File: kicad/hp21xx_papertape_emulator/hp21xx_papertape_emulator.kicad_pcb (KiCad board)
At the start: 2 copper layers, 66.5 x 61.2 mm, 85 parts, among them J1 SWD, J2 SERIAL, J3 Micro_SD_Card_Det_Hirose_DM3AT, J5 Conn_02x13_Odd_Even, SW1 Select, SW2 Up, SW3 Down, U1 TLV75533PDRV, U2 STM32F103C8Tx, U3 USBLC6-2SC6, U4 74HCT04, U5 74HCT245, U6 74LVC14, U7 74LVC245, Y1 8MHz

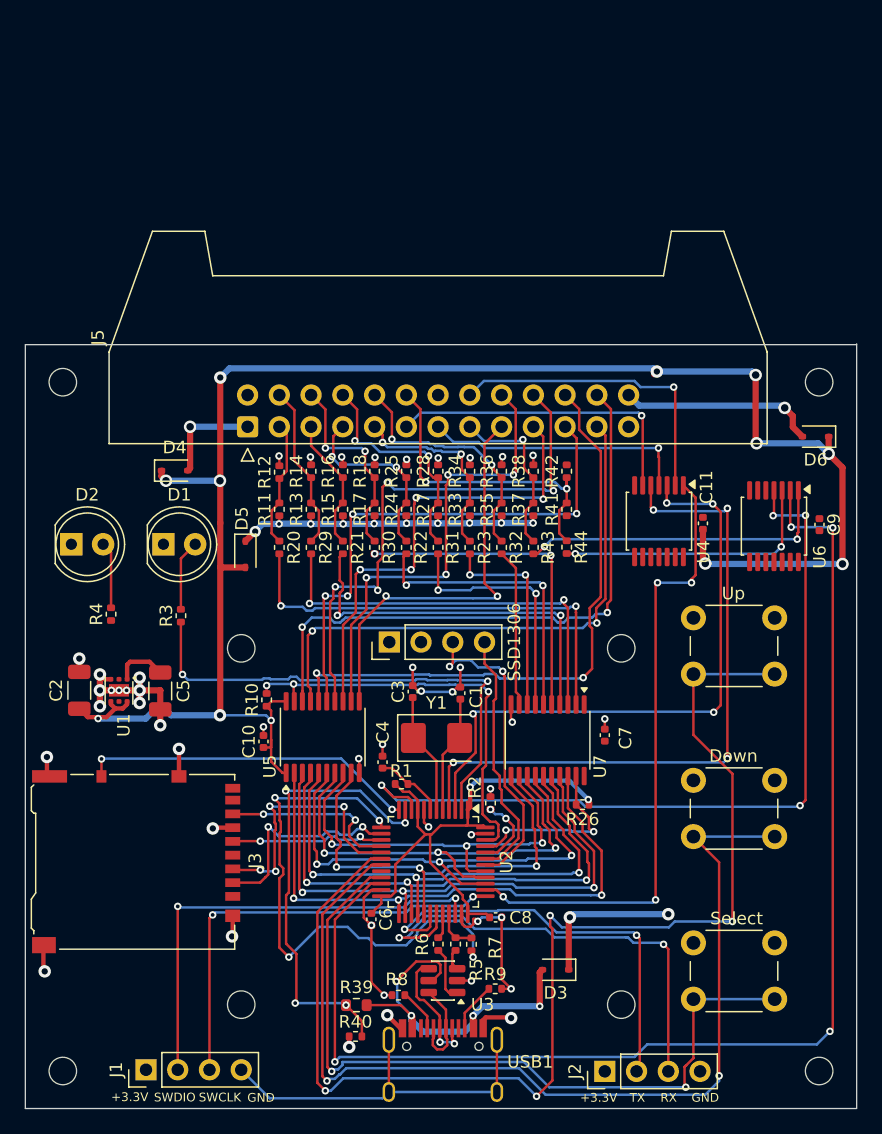
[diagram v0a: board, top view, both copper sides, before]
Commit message: New drivers.
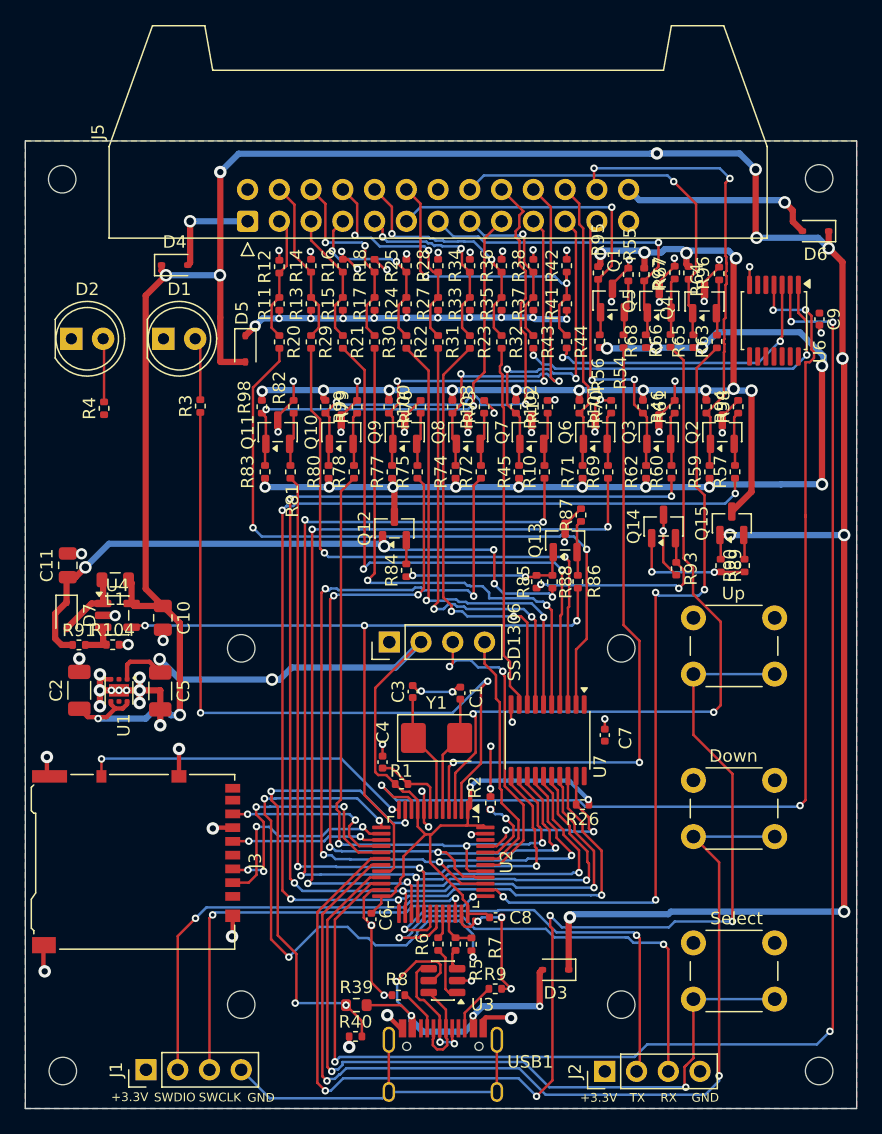
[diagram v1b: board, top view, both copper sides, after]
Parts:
- removed U5: 74HCT245, Package_SO:TSSOP-20_4.4x6.5mm_P0.65mm
- added D7: 1N5819WS, Diode_SMD:D_SOD-323, F.Cu at (92.2, 113.0)
- added L1: 10uH, Inductor_SMD:L_0805_2012Metric, F.Cu at (96.1, 110.1)
- added Q1: 2N7002, Package_TO_SOT_SMD:SOT-23, F.Cu at (135.9, 87.8)
- added Q10: 2N7002, Package_TO_SOT_SMD:SOT-23, F.Cu at (114.2, 98.3)
- added Q11: 2N7002, Package_TO_SOT_SMD:SOT-23, F.Cu at (109.1, 98.3)
- added Q12: BSS84, Package_TO_SOT_SMD:SOT-23, F.Cu at (118.4, 106.0)
- added Q13: 2N7002, Package_TO_SOT_SMD:SOT-23, F.Cu at (132.1, 107.0)
- added Q14: 2N7002, Package_TO_SOT_SMD:SOT-23, F.Cu at (140.0, 105.8)
- added Q15: BSS84, Package_TO_SOT_SMD:SOT-23, F.Cu at (145.4, 105.6)
- added Q2: 2N7002, Package_TO_SOT_SMD:SOT-23, F.Cu at (144.7, 98.3)
- added Q3: 2N7002, Package_TO_SOT_SMD:SOT-23, F.Cu at (139.6, 98.3)
- added Q4: 2N7002, Package_TO_SOT_SMD:SOT-23, F.Cu at (143.2, 87.8)
- added Q5: 2N7002, Package_TO_SOT_SMD:SOT-23, F.Cu at (139.6, 87.8)
- added Q6: 2N7002, Package_TO_SOT_SMD:SOT-23, F.Cu at (134.5, 98.3)
- added Q7: 2N7002, Package_TO_SOT_SMD:SOT-23, F.Cu at (129.4, 98.3)
- added Q8: 2N7002, Package_TO_SOT_SMD:SOT-23, F.Cu at (124.3, 98.3)
- added Q9: 2N7002, Package_TO_SOT_SMD:SOT-23, F.Cu at (119.3, 98.3)
- added R100: 1k, Resistor_SMD:R_0402_1005Metric, F.Cu at (118.0, 96.3)
- added R101: 1k, Resistor_SMD:R_0402_1005Metric, F.Cu at (133.2, 96.3)
- added R102: 1k, Resistor_SMD:R_0402_1005Metric, F.Cu at (128.1, 96.3)
- added R103: 1k, Resistor_SMD:R_0402_1005Metric, F.Cu at (123.1, 96.3)
- added R104: 10k, Resistor_SMD:R_0402_1005Metric, F.Cu at (95.9, 115.3)
- added R19: 100k, Resistor_SMD:R_0402_1005Metric, F.Cu at (130.7, 96.3)
- added R45: 10k, Resistor_SMD:R_0402_1005Metric, F.Cu at (128.4, 101.5)
- added R46: 1k, Resistor_SMD:R_0402_1005Metric, F.Cu at (138.3, 96.3)
- added R54: 100, Resistor_SMD:R_0402_1005Metric, F.Cu at (136.8, 91.0)
- added R55: 100k, Resistor_SMD:R_0402_1005Metric, F.Cu at (137.1, 85.7)
- added R56: 10k, Resistor_SMD:R_0402_1005Metric, F.Cu at (134.8, 91.0)
- added R57: 100, Resistor_SMD:R_0402_1005Metric, F.Cu at (145.7, 101.5)
- added R58: 100k, Resistor_SMD:R_0402_1005Metric, F.Cu at (145.9, 96.3)
- added R59: 10k, Resistor_SMD:R_0402_1005Metric, F.Cu at (143.6, 101.5)
- added R60: 100, Resistor_SMD:R_0402_1005Metric, F.Cu at (140.6, 101.5)
- added R61: 100k, Resistor_SMD:R_0402_1005Metric, F.Cu at (140.8, 96.3)
- added R62: 10k, Resistor_SMD:R_0402_1005Metric, F.Cu at (138.6, 101.5)
- added R63: 100, Resistor_SMD:R_0402_1005Metric, F.Cu at (144.2, 91.0)
- added R64: 100k, Resistor_SMD:R_0402_1005Metric, F.Cu at (144.4, 85.6)
- added R65: 10k, Resistor_SMD:R_0402_1005Metric, F.Cu at (142.3, 91.0)
- added R66: 100, Resistor_SMD:R_0402_1005Metric, F.Cu at (140.5, 91.0)
- added R67: 100k, Resistor_SMD:R_0402_1005Metric, F.Cu at (140.8, 85.5)
- added R68: 10k, Resistor_SMD:R_0402_1005Metric, F.Cu at (138.5, 91.0)
- added R69: 100, Resistor_SMD:R_0402_1005Metric, F.Cu at (135.5, 101.5)
- added R70: 100k, Resistor_SMD:R_0402_1005Metric, F.Cu at (135.8, 96.3)
- added R71: 10k, Resistor_SMD:R_0402_1005Metric, F.Cu at (133.5, 101.5)
- added R72: 100, Resistor_SMD:R_0402_1005Metric, F.Cu at (125.3, 101.5)
- added R73: 100k, Resistor_SMD:R_0402_1005Metric, F.Cu at (125.6, 96.3)
- added R74: 10k, Resistor_SMD:R_0402_1005Metric, F.Cu at (123.3, 101.5)
- added R75: 100, Resistor_SMD:R_0402_1005Metric, F.Cu at (120.3, 101.5)
- added R76: 100k, Resistor_SMD:R_0402_1005Metric, F.Cu at (120.5, 96.3)
- added R77: 10k, Resistor_SMD:R_0402_1005Metric, F.Cu at (118.2, 101.5)
- added R78: 100, Resistor_SMD:R_0402_1005Metric, F.Cu at (115.2, 101.5)
- added R79: 100k, Resistor_SMD:R_0402_1005Metric, F.Cu at (115.4, 96.3)
- added R80: 10k, Resistor_SMD:R_0402_1005Metric, F.Cu at (113.2, 101.5)
- added R81: 100, Resistor_SMD:R_0402_1005Metric, F.Cu at (110.1, 101.5)
- added R82: 100k, Resistor_SMD:R_0402_1005Metric, F.Cu at (110.4, 96.3)
- added R83: 10k, Resistor_SMD:R_0402_1005Metric, F.Cu at (108.1, 101.5)
- added R84: 100, Resistor_SMD:R_0402_1005Metric, F.Cu at (119.4, 109.3)
- added R85: 100k, Resistor_SMD:R_0402_1005Metric, F.Cu at (131.1, 110.3)
- added R86: 100, Resistor_SMD:R_0402_1005Metric, F.Cu at (133.1, 110.3)
- added R87: 100k, Resistor_SMD:R_0402_1005Metric, F.Cu at (133.3, 104.9)
- added R88: 100, Resistor_SMD:R_0402_1005Metric, F.Cu at (129.8, 110.3)
- added R89: 100k, Resistor_SMD:R_0402_1005Metric, F.Cu at (144.5, 109.0)
- added R90: 100, Resistor_SMD:R_0402_1005Metric, F.Cu at (146.4, 109.0)
- added R91: 86.6k, Resistor_SMD:R_0402_1005Metric, F.Cu at (93.2, 115.3)
- added R93: 100k, Resistor_SMD:R_0402_1005Metric, F.Cu at (141.0, 109.2)
- added R94: 1k, Resistor_SMD:R_0402_1005Metric, F.Cu at (143.4, 96.3)
- added R95: 1k, Resistor_SMD:R_0402_1005Metric, F.Cu at (134.7, 85.6)
- added R96: 1k, Resistor_SMD:R_0402_1005Metric, F.Cu at (142.0, 85.6)
- added R97: 1k, Resistor_SMD:R_0402_1005Metric, F.Cu at (138.4, 85.7)
- added R98: 1k, Resistor_SMD:R_0402_1005Metric, F.Cu at (107.8, 96.3)
- added R99: 1k, Resistor_SMD:R_0402_1005Metric, F.Cu at (112.9, 96.3)
- C10, C11: value 100n -> 1u; footprint Capacitor_SMD:C_0402_1005Metric -> Capacitor_SMD:C_0805_2012Metric
- R10: value 100k -> 100
- U4: value 74HCT04 -> AP3012; footprint Package_SO:TSSOP-14_4.4x5mm_P0.65mm -> Package_TO_SOT_SMD:SOT-23-5
- moved C11 50.9 mm to (92.3, 109.0)
- moved U4 44.0 mm to (96.3, 113.0), turned to 0 degrees
- moved R10 28.7 mm to (130.4, 101.5)
- moved R3 16.8 mm to (102.9, 96.2)
- moved R4 16.5 mm to (95.2, 96.4)
- moved D1 16.4 mm to (99.9, 90.8)
- moved D2 16.4 mm to (92.6, 90.8)
- moved J5 16.4 mm to (106.7, 81.4)
- moved R11 16.4 mm to (109.2, 88.0)
- moved R23 16.4 mm to (124.5, 91.1)
- moved R27 16.4 mm to (121.9, 88.0)
- moved R35 16.4 mm to (127.0, 88.0)
- moved R37 16.4 mm to (129.5, 88.0)
- moved R41 16.4 mm to (132.2, 88.0)
- moved U6 16.4 mm to (148.8, 89.4)
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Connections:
- C11 pad 1: +5V -> +12V
- R10 pad 1: +5V -> /D3
- R10 pad 2: /RDREN -> Net-(Q7-G)
- U2 pad 20: unconnected-(U2-PB2-Pad20) -> /PUSEL
- U2 pad 46: /RDREN -> unconnected-(U2-PB9-Pad46)
- U4 pad 1: /FLAG_PTR -> Net-(D7-A)
- U4 pad 2: /OUTFR -> GND
- U4 pad 3: /PAPEROUT -> Net-(U4-FB)
- U4 pad 4: /PAPER_LOW -> /PUSEL
- U4 pad 5: /FLAG_PTP -> +5V
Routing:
- net /PU12V: track 0.00 -> 83.9 mm, vias 0 -> 13
- net /PU5V: track 0.00 -> 81.9 mm, vias 0 -> 14
- net +5V: track 155.1 -> 225.2 mm
- net /PUSEL: track 0.00 -> 60.0 mm, vias 0 -> 3
- net /D0: track 47.1 -> 106.6 mm, vias 3 -> 5
- net GND: track 105.5 -> 162.2 mm, vias 46 -> 74
- net /D1: track 45.5 -> 99.5 mm, vias 3 -> 5
- net +12V: track 0.00 -> 50.9 mm, vias 0 -> 5
- net /D2: track 44.2 -> 91.1 mm, vias 3 -> 5
- net /D3: track 42.1 -> 85.8 mm, vias 3 -> 5
- net +3.3V: track 46.7 -> 84.5 mm, vias 2 -> 4
- net /D4: track 40.6 -> 75.8 mm, vias 3 -> 5
- net /RDREN: track 34.0 -> 0.00 mm, vias 3 -> 0
- net /D5: track 37.5 -> 66.9 mm, vias 3 -> 5
- net /D7: track 36.6 -> 62.7 mm
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- added copper zone on F.Cu, net +3.3V
- added copper zone on B.Cu, net GND
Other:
- board size 66.5 x 61.2 mm -> 66.5 x 77.4 mm
